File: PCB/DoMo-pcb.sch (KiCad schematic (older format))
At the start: 4 parts, among them SW0 SW_Push, SW1 Rotary_Encoder_Switch, U0 ProMicro

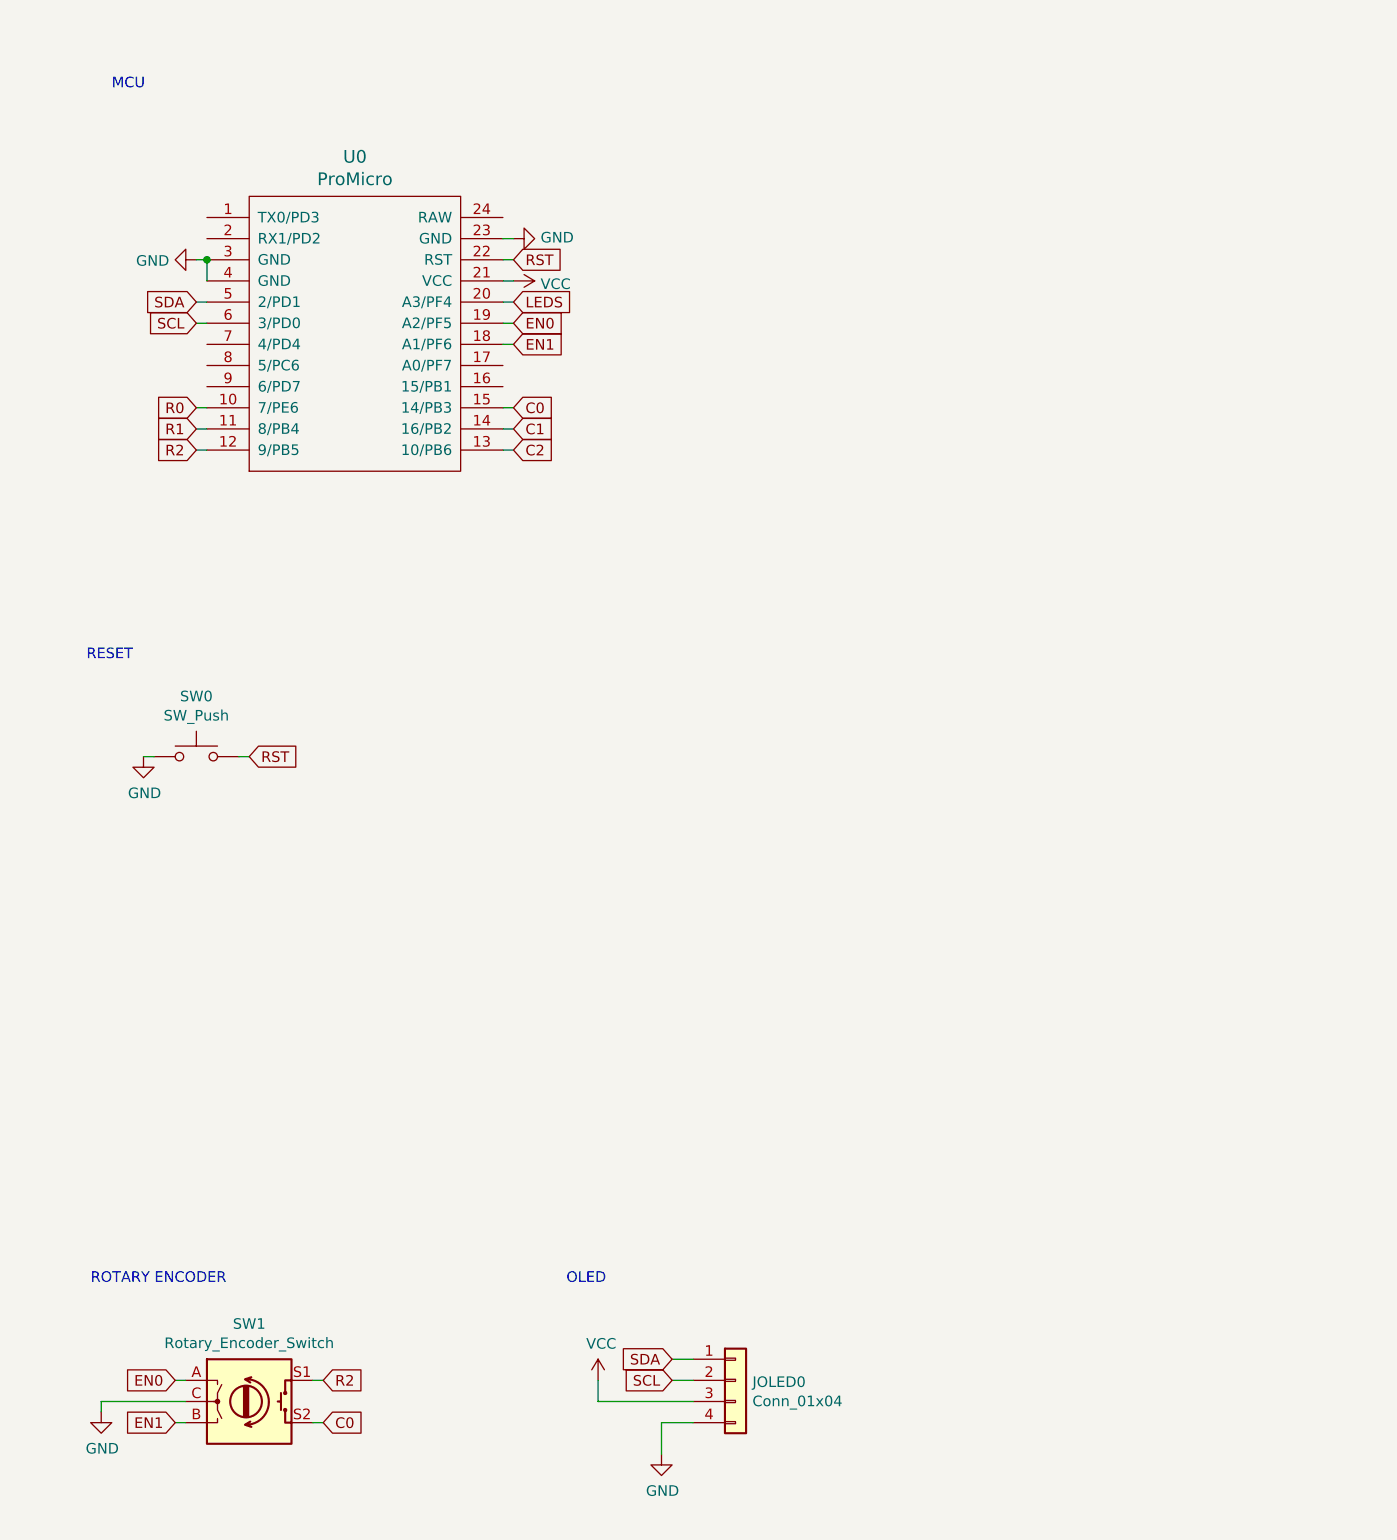
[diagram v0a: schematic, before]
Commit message: create LEDS
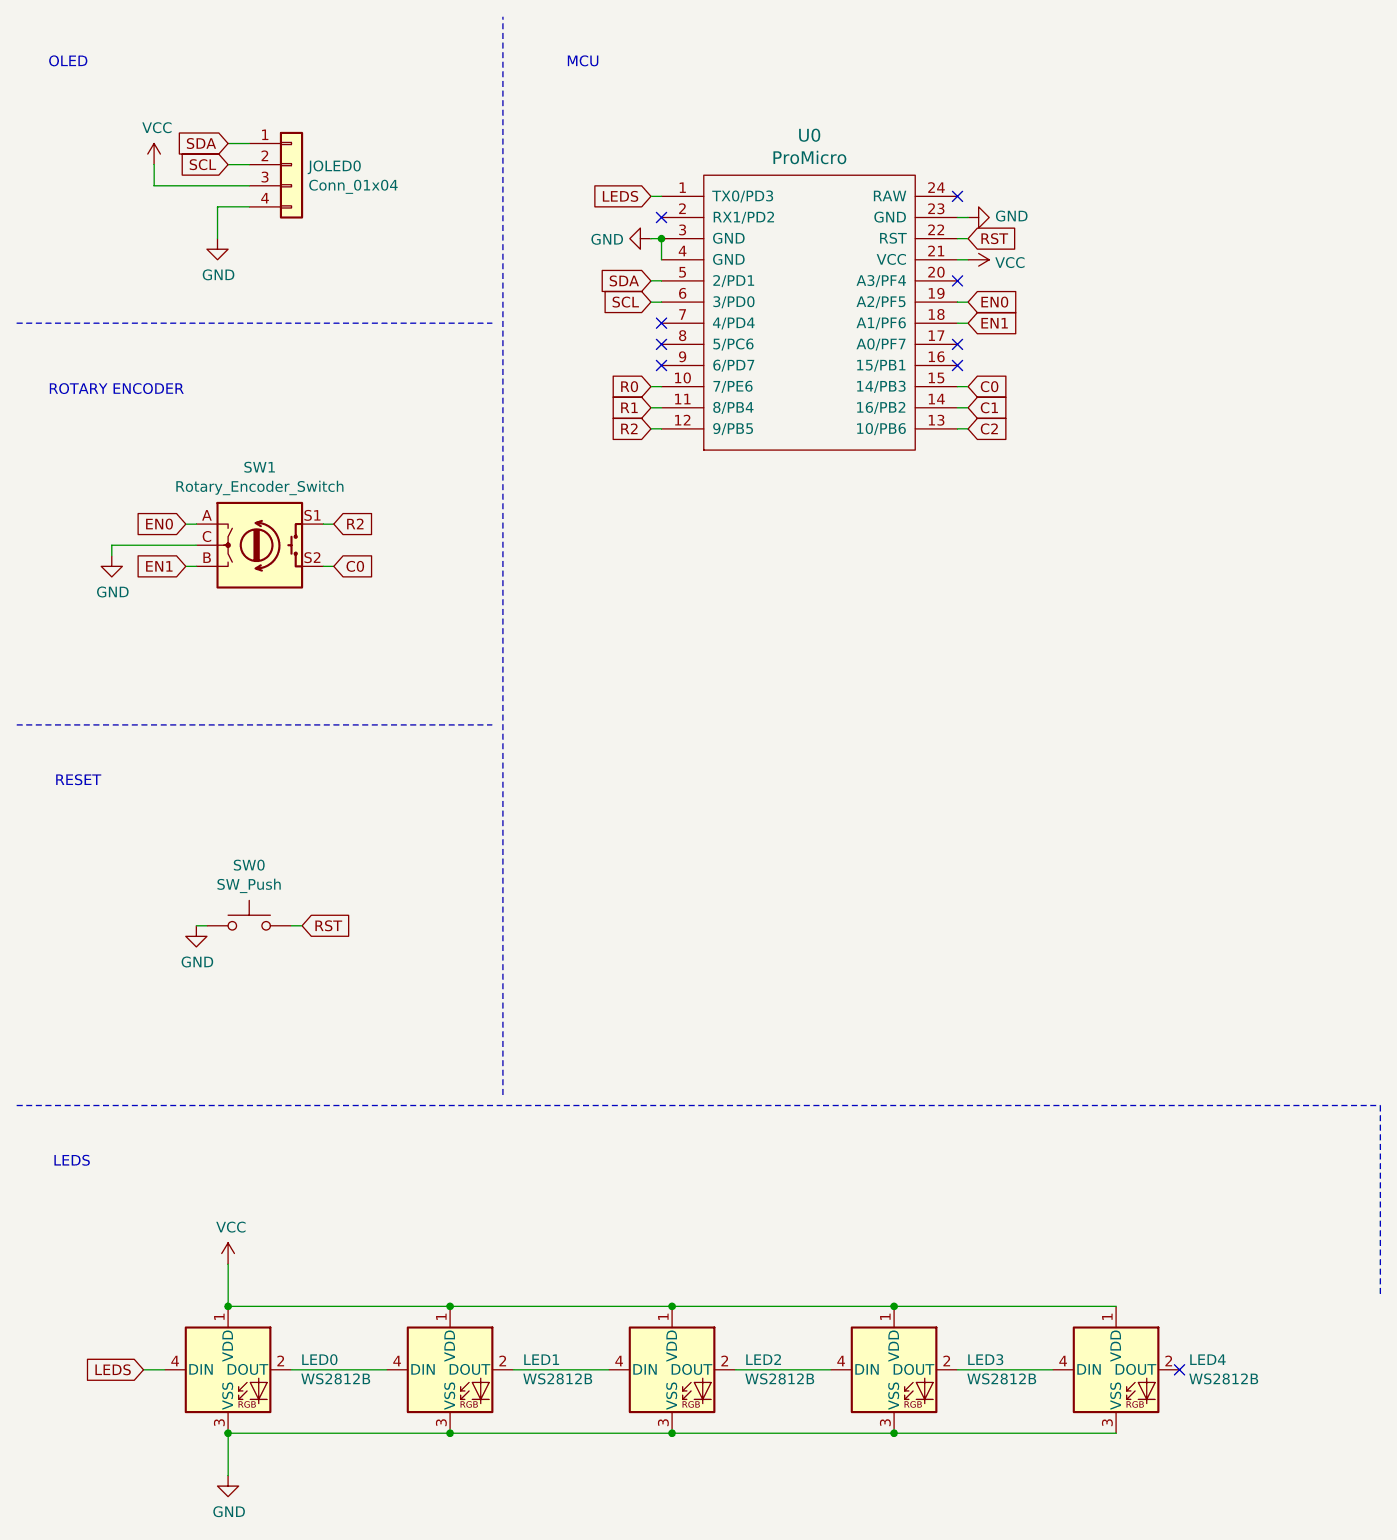
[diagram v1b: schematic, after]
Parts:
- added LED0, LED1, LED2, LED3, LED4: WS2812B, LED_SMD:LED_WS2812B_PLCC4_5.0x5.0mm_P3.2mm, symbol LED:WS2812B
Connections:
- net GND: now also LED0.3 (VSS), LED1.3 (VSS), LED2.3 (VSS), LED3.3 (VSS), LED4.3 (VSS)
- net LEDS: now also U0.1 (TX0/PD3), LED0.4 (DIN); no longer U0.20 (A3/PF4)
- net VCC: now also LED0.1 (VDD), LED1.1 (VDD), LED2.1 (VDD), LED3.1 (VDD), LED4.1 (VDD)
- new net: LED0.2 (DOUT), LED1.4 (DIN)
- new net: LED1.2 (DOUT), LED2.4 (DIN)
- new net: LED2.2 (DOUT), LED3.4 (DIN)
- new net: LED3.2 (DOUT), LED4.4 (DIN)
- no-connect marks 0 -> 9
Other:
- note added: "LEDS"
- moved on the sheet: JOLED0, SW0, SW1, U0
